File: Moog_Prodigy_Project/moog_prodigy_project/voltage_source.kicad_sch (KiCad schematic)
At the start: 24 parts, among them T2 230 VAC/ 15VAC 1A5 22W, U24 LM78L12, U25 LM79L12

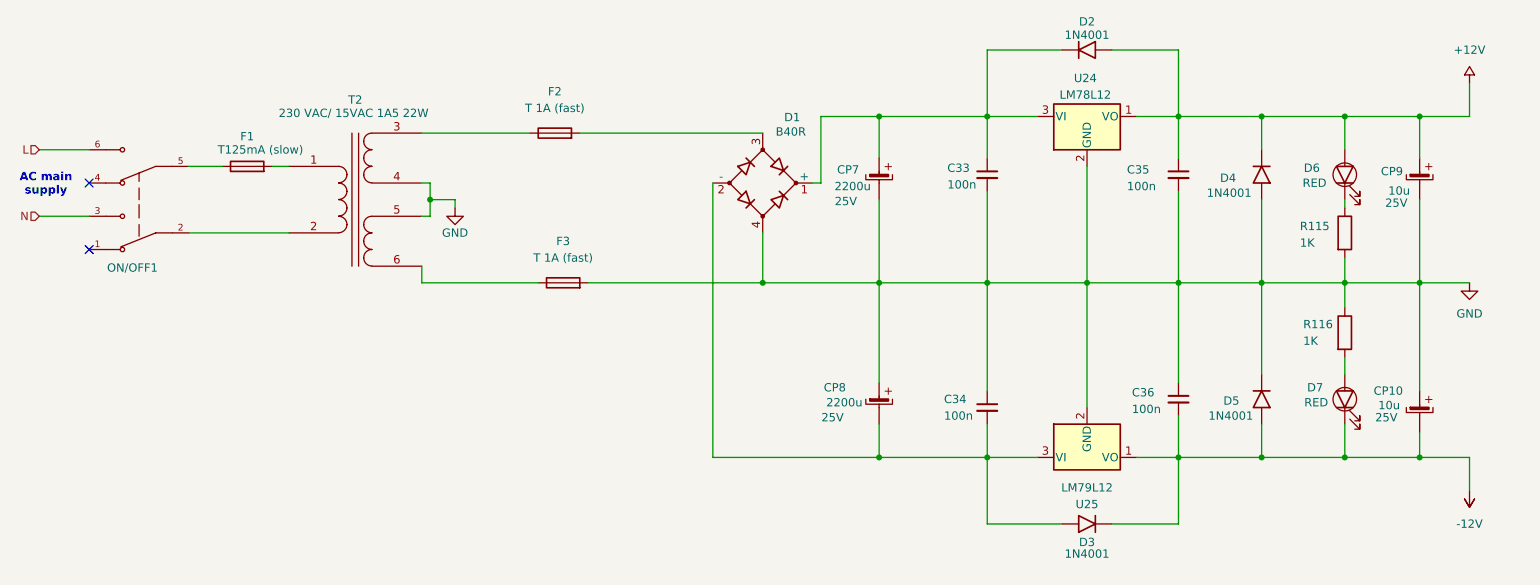
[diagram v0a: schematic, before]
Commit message: 07.06.2026 fix 3
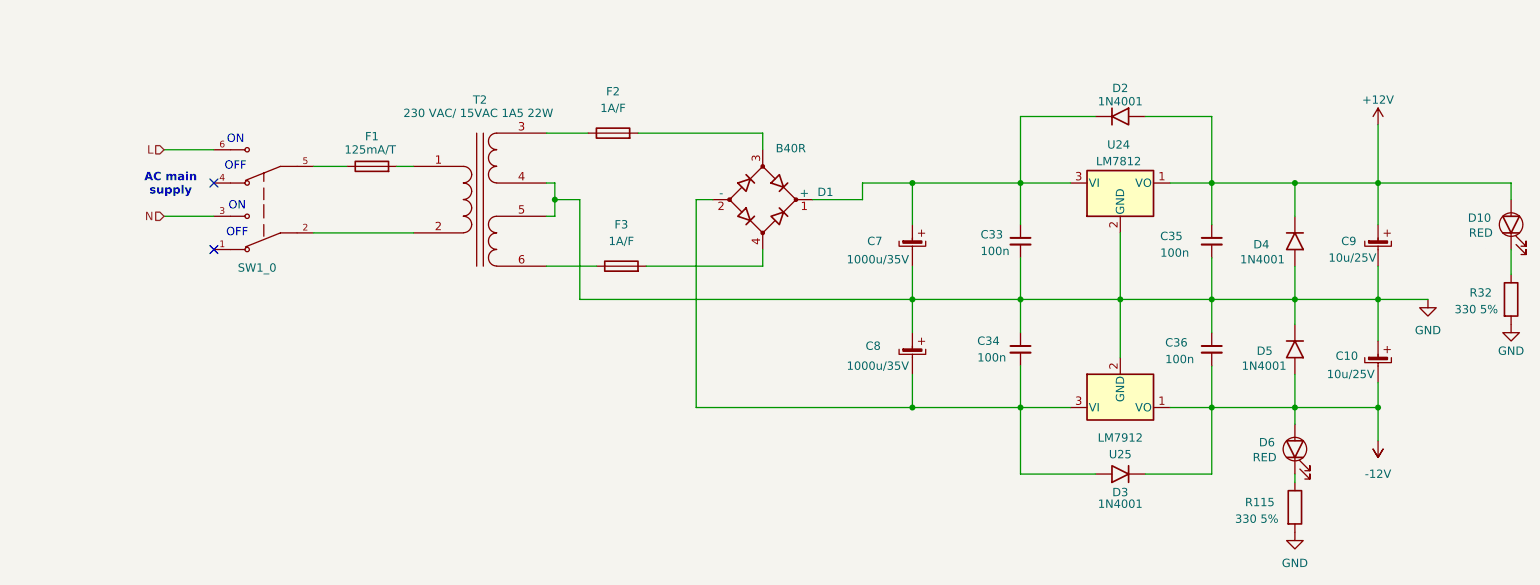
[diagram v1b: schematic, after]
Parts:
- removed D7: RED, symbol Device:LED
- removed R116: 1K, symbol Device:R
- added D10: RED, symbol Device:LED
- added R32: 330 5%, symbol Device:R
- C10: renamed from CP10; value 10u -> 10u/25V
- C7: renamed from CP7; value 2200u -> 1000u/35V; Rated Voltage 25V -> 35V
- C8: renamed from CP8; value 2200u -> 1000u/35V; Rated Voltage 25V -> 35V
- C9: renamed from CP9; value 10u -> 10u/25V
- F1: value T125mA (slow) -> 125mA/T
- F2, F3: value T 1A (fast) -> 1A/F
- R115: value 1K -> 330 5%
- U24: value LM78L12 -> LM7812
- U25: value LM79L12 -> LM7912
- renumbered ON/OFF1 to SW1_0
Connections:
- net +12V: now also D10.2 (A); no longer D6.2 (A)
- net -12V: now also D6.2 (A)
- net GND: now also R32.2; no longer D1.4, F3.2
- new net: D1.4, F3.2
- new net: D10.1 (K), R32.1
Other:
- note added: "ON OFF"
- moved on the sheet: C10, C33, C34, C35, C36, C7, C8, C9, D1, D2, D3, D4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
